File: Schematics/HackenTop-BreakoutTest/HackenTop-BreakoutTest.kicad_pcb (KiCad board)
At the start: 2 copper layers, 45 parts, among them J1 USB_B_Micro, J2 Conn_01x07, J3 HDMI_A, J4 Conn_01x03, J5 Conn_01x25, J6 Conn_01x21, J7 CONN_1473005-1_TYCO, J8 Power, Q1 2N7002, Q2 2N7002, Q3 2N7002, Q4 2N7002, U1 TLV1117-33, U2 MIC5504-1.8YM5, U3 ESD5384, U4 AP2331W, U5 LT1963AxST-2.5

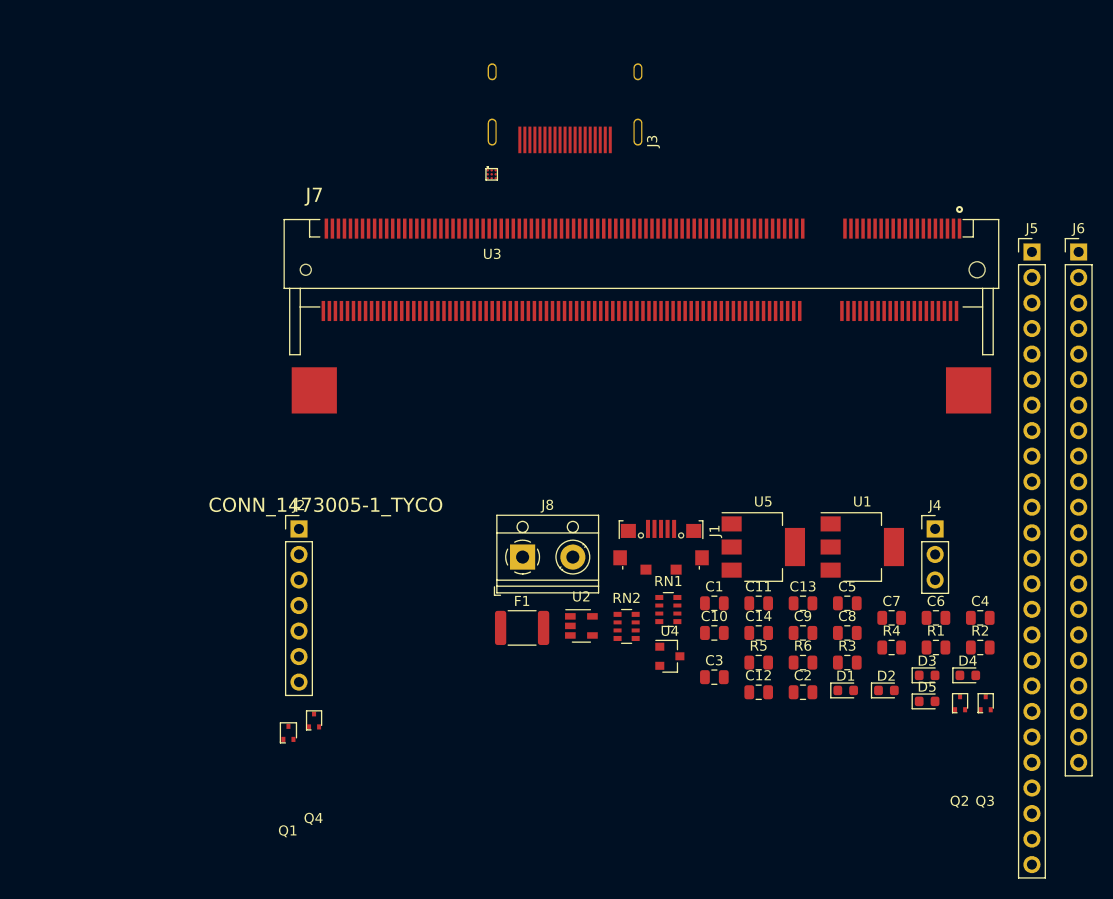
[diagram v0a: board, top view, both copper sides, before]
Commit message: V1 ordered May26
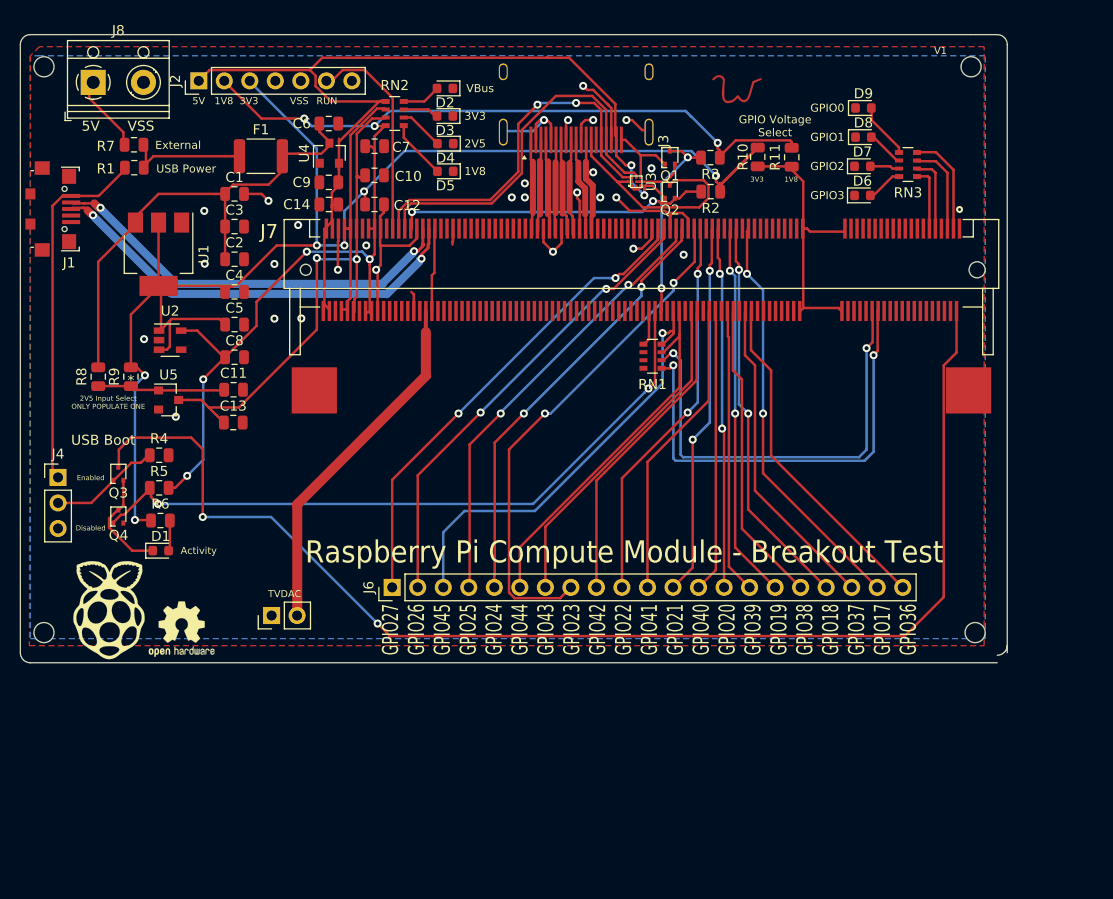
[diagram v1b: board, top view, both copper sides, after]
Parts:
- removed J5: Conn_01x25, Connector_PinHeader_2.54mm:PinHeader_1x25_P2.54mm_Vertical
- added D6: LED_Small, LED_SMD:LED_0603_1608Metric, F.Cu at (197.8, 55.9)
- added D7: LED_Small, LED_SMD:LED_0603_1608Metric, F.Cu at (197.8, 53.0)
- added D8: LED_Small, LED_SMD:LED_0603_1608Metric, F.Cu at (197.9, 50.1)
- added D9: LED_Small, LED_SMD:LED_0603_1608Metric, F.Cu at (197.9, 47.2)
- added R10: 0ohm, Resistor_SMD:R_0805_2012Metric, F.Cu at (187.4, 52.1)
- added R11: 0ohm, Resistor_SMD:R_0805_2012Metric, F.Cu at (190.8, 52.1)
- added R7: 0ohm, Resistor_SMD:R_0805_2012Metric, F.Cu at (125.3, 50.9)
- added R8: 0ohm, Resistor_SMD:R_0805_2012Metric, F.Cu at (121.8, 73.9)
- added R9: 0ohm, Resistor_SMD:R_0805_2012Metric, F.Cu at (125.0, 73.9)
- added REF**: MountingHole_2mm, MountingHole:MountingHole_2mm, F.Cu at (116.3, 99.4)
- added REF**: MountingHole_2mm, MountingHole:MountingHole_2mm, F.Cu at (116.3, 43.1)
- added REF**: MountingHole_2mm, MountingHole:MountingHole_2mm, F.Cu at (208.6, 43.1)
- added REF**: MountingHole_2mm, MountingHole:MountingHole_2mm, F.Cu at (209.0, 99.4)
- added REF**: OSHW-Logo2_7.3x6mm_SilkScreen, Symbol:OSHW-Logo2_7.3x6mm_SilkScreen, F.Cu at (130.1, 99.0)
- added RN3: 470ohm, Resistor_SMD:R_Array_Convex_4x0603, F.Cu at (202.3, 52.8)
- added Ref**: Val**, HackenTop:raspberry, F.Cu at (122.8, 97.2)
- added Ref**: Val**, NFCBuisness:W, F.Cu at (185.3, 46.4)
- added TVDAC: PinHeader_1x02_P2.54mm_Vertical, Connector_PinHeader_2.54mm:PinHeader_1x02_P2.54mm_Vertical, F.Cu at (139.0, 97.7)
- U5: footprint Package_TO_SOT_SMD:SOT-223-3_TabPin2 -> Package_TO_SOT_SMD:SOT-23
- moved R1 93.0 mm to (125.3, 53.1)
- moved Q3 89.3 mm to (123.8, 84.2)
- moved J4 87.4 mm to (117.8, 84.0)
- moved C4 81.0 mm to (135.3, 65.5)
- moved C6 77.9 mm to (144.7, 48.8)
- moved J6 76.0 mm to (151.0, 94.9), turned to 90 degrees
- moved U1 75.8 mm to (127.8, 61.8), turned to 270 degrees
- moved R4 75.4 mm to (127.8, 81.8)
- moved D2 74.3 mm to (156.2, 45.2), turned to 180 degrees
- moved D4 74.2 mm to (156.3, 50.8), turned to 180 degrees
- moved D3 73.5 mm to (156.2, 48.0), turned to 180 degrees
- moved D5 71.3 mm to (156.3, 53.5), turned to 180 degrees
- moved C2 71.1 mm to (135.3, 62.2)
- moved C7 69.6 mm to (149.2, 51.0), turned to 180 degrees
- moved J1 69.6 mm to (117.0, 57.2), turned to 270 degrees
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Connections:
- C11 pad 1: VBUS -> Net-(C11-Pad1)
- C14 pad 2: VBUS -> +5V
- F1 pad 1: +5VA -> Net-(F1-Pad1)
- F1 pad 2: Net-(F1-Pad2) -> VBUS
- J1 pad 1: Net-(F1-Pad2) -> +5VA
- J1 pad 4: USB_OTGID -> Net-(J1-Pad4)
- J2 pad 1: VBUS -> +5V
- J3 pad 20: (no net) -> VSS
- J3 pad 21: (no net) -> VSS
- J3 pad 22: (no net) -> VSS
- J3 pad 23: (no net) -> VSS
- J6 pad 5: GPIO44 -> GPIO24
- J6 pad 6: GPIO24 -> GPIO44
- J7 pad 197: VBUS -> +5V
- J7 pad 198: VBUS -> +5V
- J7 pad 199: VBUS -> +5V
- J7 pad 200: VBUS -> +5V
- J7 pad 41: GPIO28-45_VDD -> GPIO0-27_VDD
- J7 pad 42: GPIO28-45_VDD -> GPIO0-27_VDD
- J7 pad SH1: (no net) -> VSS
- J7 pad SH2: (no net) -> VSS
- J8 pad 1: VBUS -> +BATT
- R1 pad 2: VBUS -> Net-(F1-Pad1)
- RN2 pad 1: VBUS -> +5V
- U5 pad 1: VBUS -> Net-(C11-Pad1)
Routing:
- net +3V3: track 0.00 -> 171.5 mm, vias 0 -> 6
- net EMMC_DISABLE_N: track 0.00 -> 127.1 mm, vias 0 -> 2
- net +1V8: track 0.00 -> 127.0 mm, vias 0 -> 7
- net +5V: track 0.00 -> 94.7 mm, vias 0 -> 2
- net VSS: track 0.00 -> 90.7 mm, vias 0 -> 28
- net EMMC_EN_N_1V8: track 0.00 -> 68.7 mm, vias 0 -> 2
- net +2V5: track 0.00 -> 52.6 mm, vias 0 -> 2
- net GPIO23: track 0.00 -> 51.0 mm, vias 0 -> 2
- net VBUS: track 0.00 -> 48.1 mm
- net GPIO27: track 0.00 -> 48.1 mm, vias 0 -> 2
- net GPIO26: track 0.00 -> 46.3 mm, vias 0 -> 2
- net GPIO28: track 0.00 -> 45.1 mm, vias 0 -> 2
- net GPIO29: track 0.00 -> 44.9 mm, vias 0 -> 2
- net GPIO25: track 0.00 -> 44.3 mm, vias 0 -> 2
- net GPIO24: track 0.00 -> 43.4 mm, vias 0 -> 2
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- added copper zone on B.Cu, net VSS
- added copper zone on F.Cu, net VSS
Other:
- board outline added: 98.2 x 62.5 mm
- net class Default: clearance 0.2 -> 0.1
- rule trace_clearance: 0.2 -> 0.1
- board text added: "*"
- board text added: "1V8"
- board text added: "2V5"
- board text added: "2V5 Input Select ONLY POPULATE ONE"
- board text added: "3V3"
- board text added: "5V"
- board text added: "Activity"
- board text added: "Disabled"
- board text added: "Enabled"
- board text added: "External"
- board text added: "GPIO Voltage Select"
- board text added: "GPIO0"
- board text added: "GPIO1"
- board text added: "GPIO2"
- board text added: "GPIO27 GPIO26 GPIO45 GPIO25 GPIO24 GPIO44 GPIO43 GPIO23 GPIO42 GPIO22 GPIO41 GPIO21 GPIO40 GPIO20 GPIO39 GPIO19 GPIO38 GPIO18 GPIO37 GPIO17 GPIO36"
- board text added: "GPIO3"
- board text added: "RUN"
- board text added: "Raspberry Pi Compute Module - Breakout Test"
- board text added: "USB Boot"
- board text added: "USB Power"
- board text added: "V1"
- board text added: "VBus"
- board text added: "VSS"
